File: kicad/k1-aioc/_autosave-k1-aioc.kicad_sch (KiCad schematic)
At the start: 46 parts, among them J1 HX TYPE-C 24P QCHT, J2 Conn_01x07_Male, Q1 BC847BS, U1 MIC5330-SSYML-TR, U2 STM32F302CBT6, Y1 8MHz/20pF

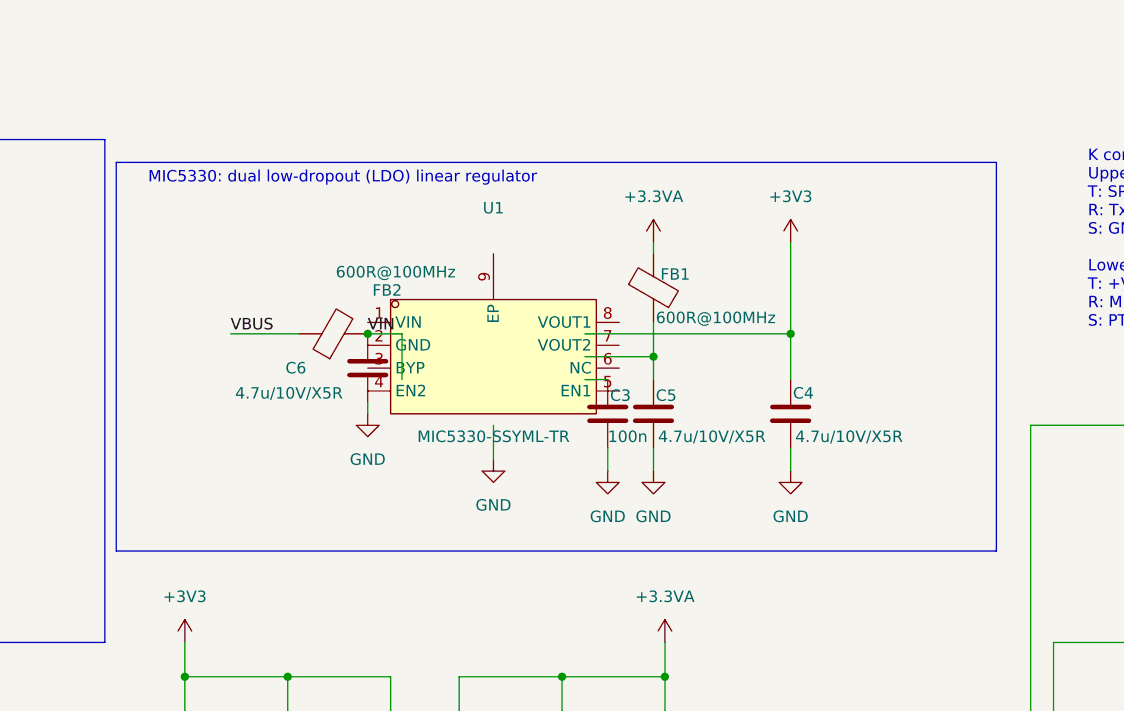
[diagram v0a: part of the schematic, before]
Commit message: tweaks
Tweaks and changes.
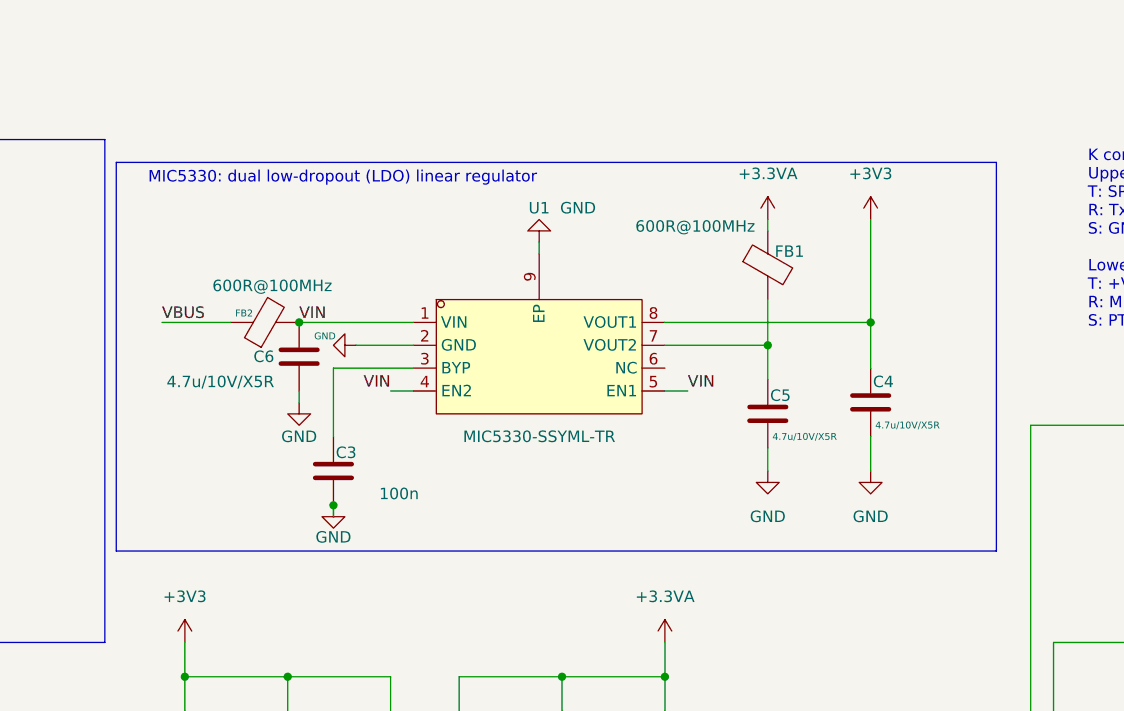
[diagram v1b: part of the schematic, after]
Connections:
- net +3V3: now also U1.8 (VOUT1)
- net GND: now also U1.2 (GND), U1.9 (EP)
- net VIN: now also U1.1 (VIN), U1.4 (EN2), U1.5 (EN1)
- net at C5.1, FB1.2: now also U1.7 (VOUT2)
- net at U1.3 (BYP): now also C3.1
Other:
- moved on the sheet: C3, C4, C5, C6, FB1, FB2, U1
